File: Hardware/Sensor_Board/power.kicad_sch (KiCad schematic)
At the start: 25 parts, among them U201 TPS7A20L_1V2, U202 TPS7A20L_2V2, U203 TPS7A20L_3V3, U204 TLV840, U301 ICE40UL1K-CM36AI

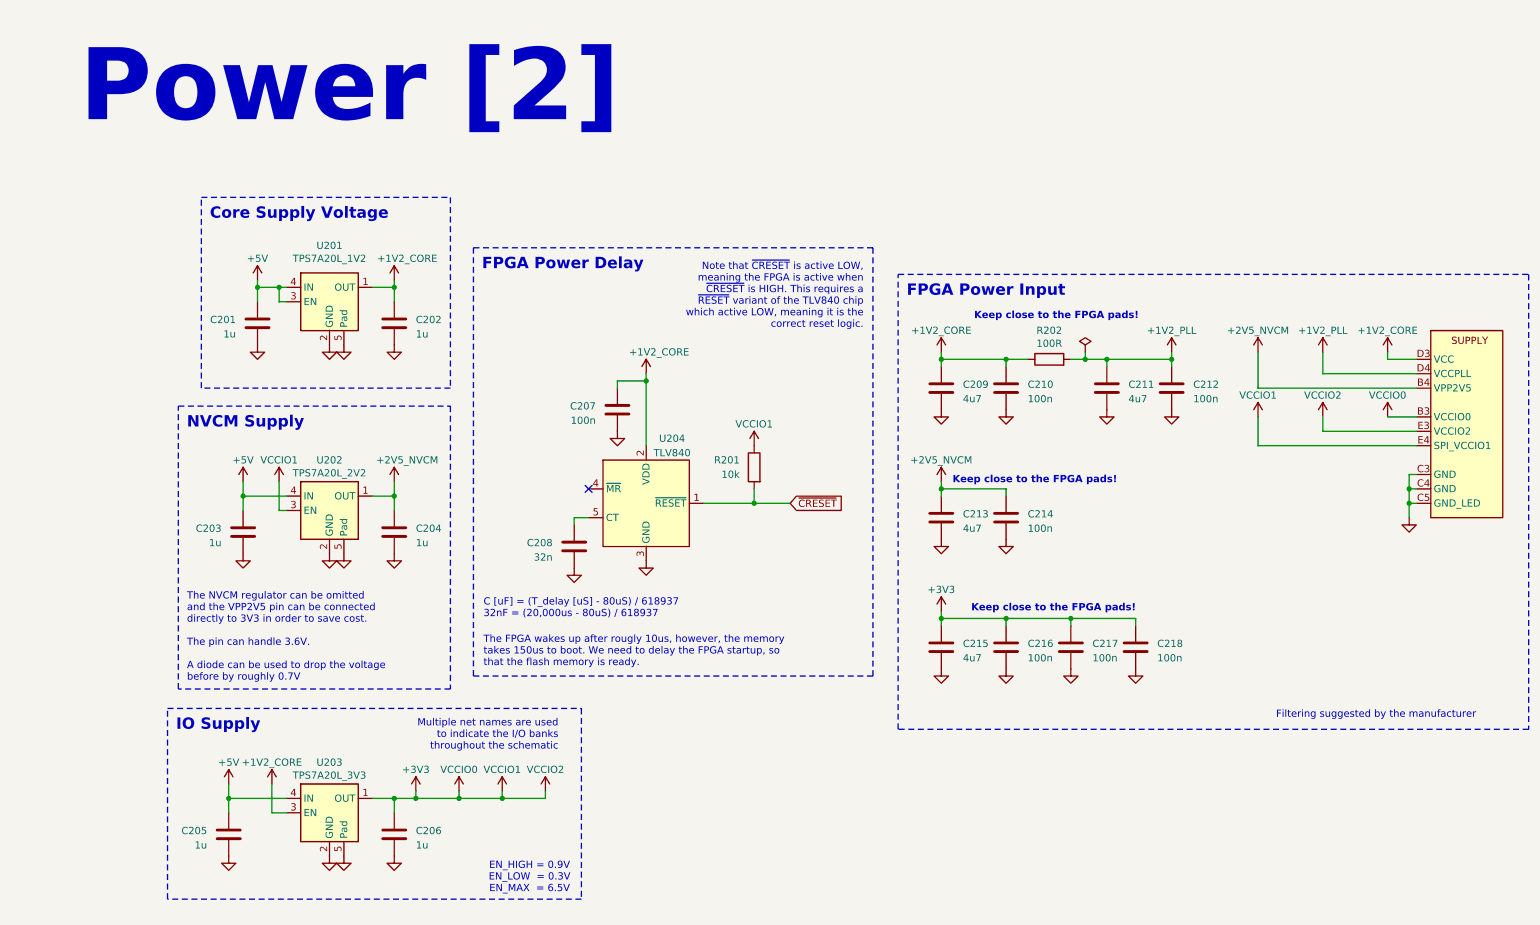
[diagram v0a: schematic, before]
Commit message: Added a programmer schematic
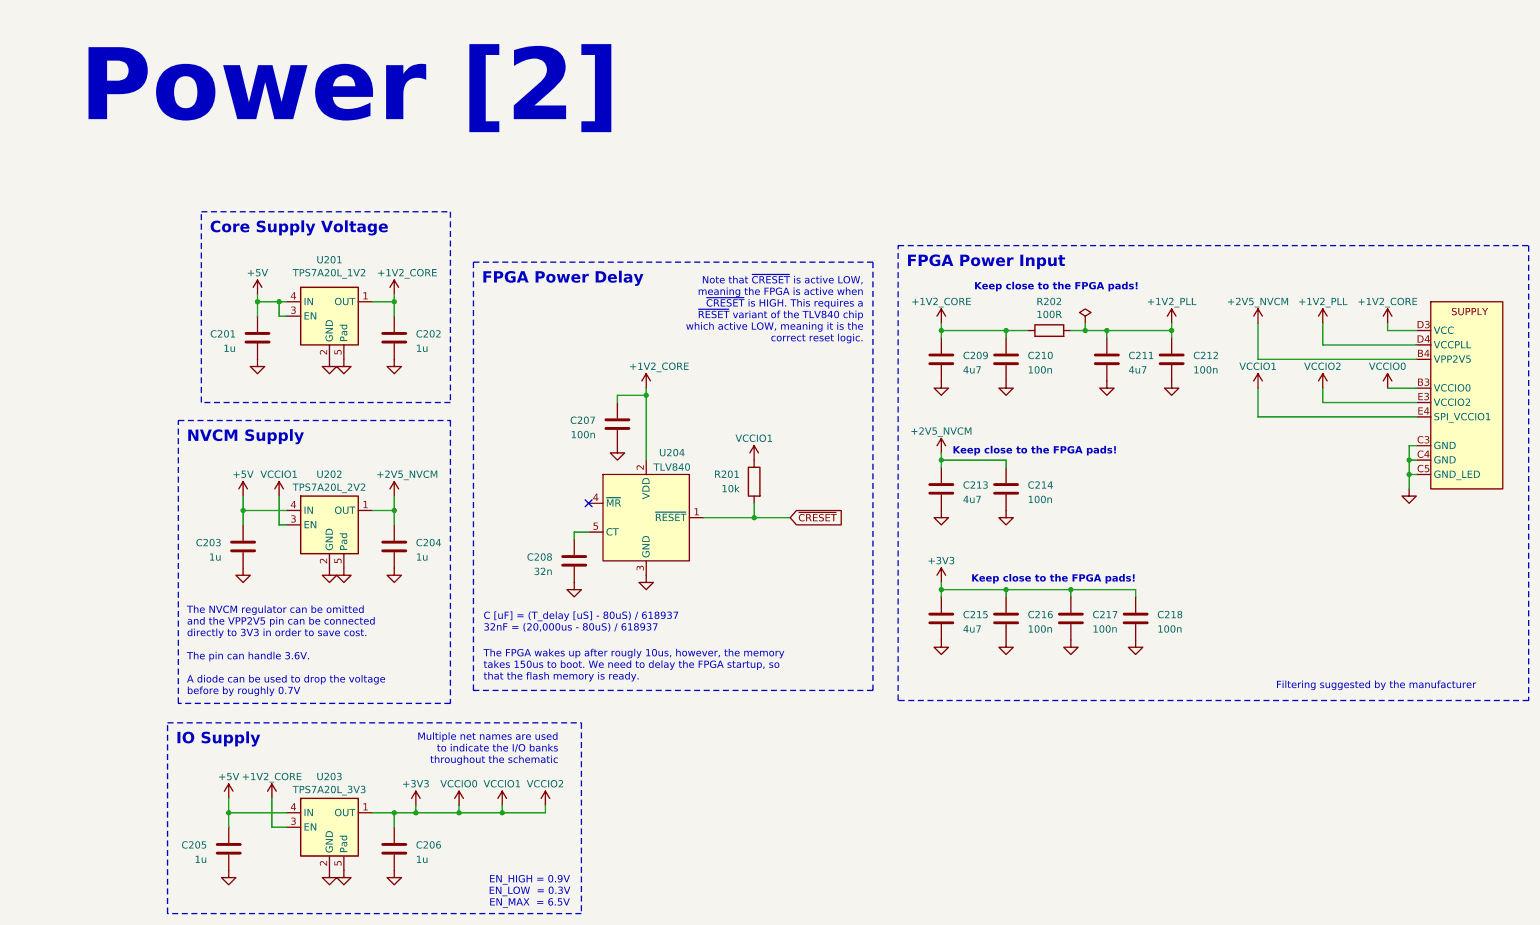
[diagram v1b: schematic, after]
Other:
- moved on the sheet: C201, C202, C203, C204, C205, C206, C207, C208, C209, C210, C211, C212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
